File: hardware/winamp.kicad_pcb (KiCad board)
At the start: 2 copper layers, 2.1 x 1.7 mm, 13 parts, among them U101 TLV271QDBVRQ1, U102 ZXBM5210-SP

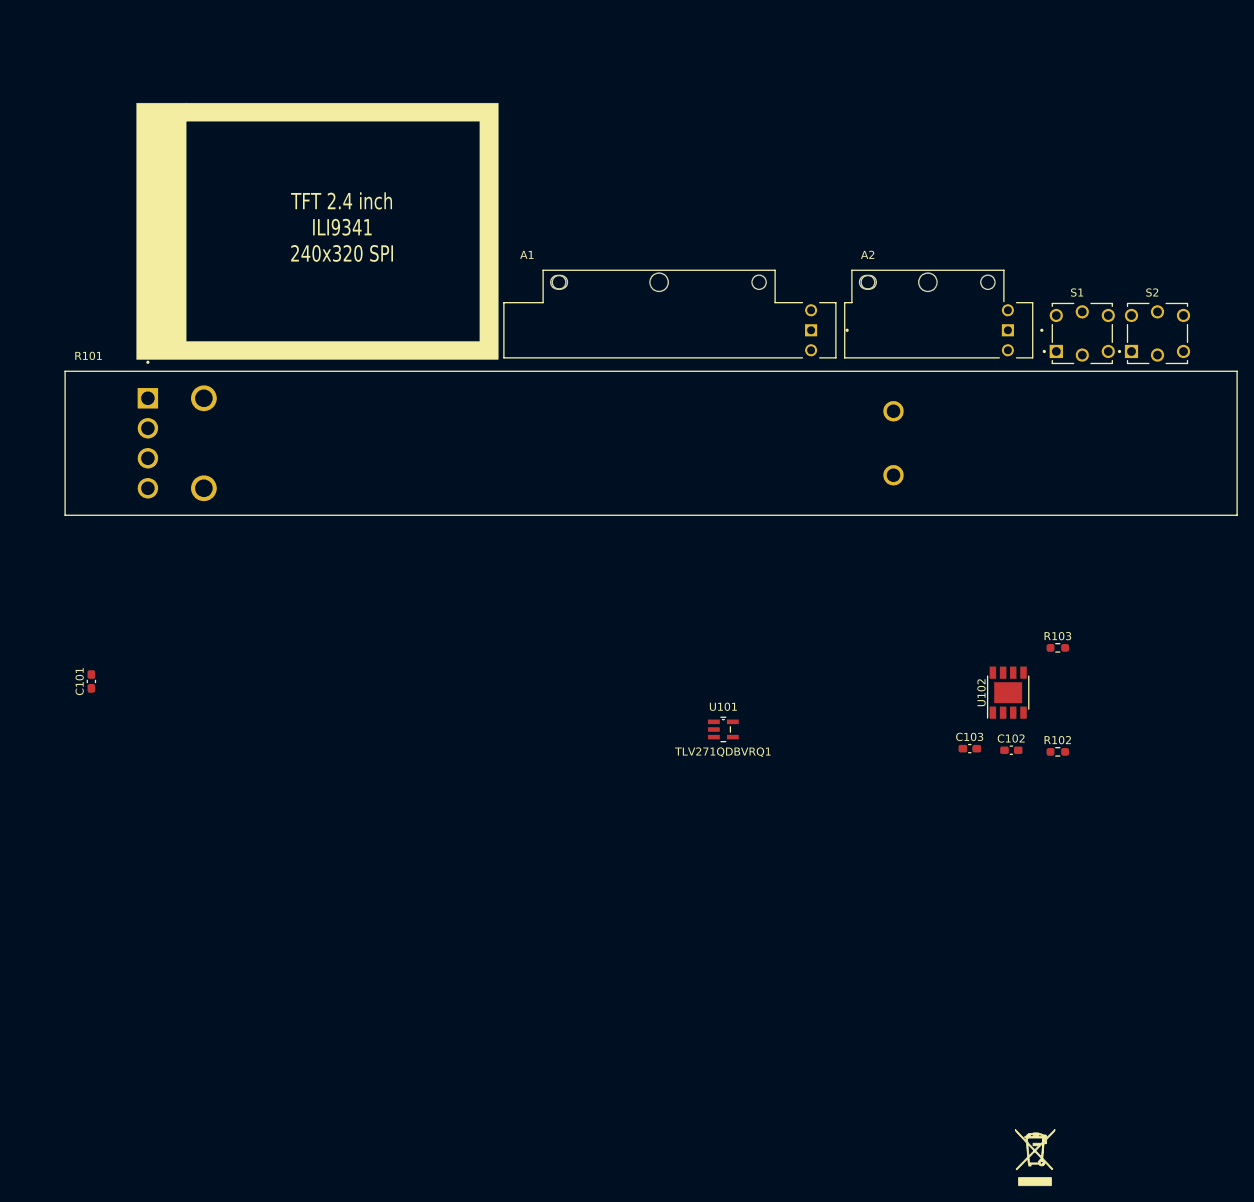
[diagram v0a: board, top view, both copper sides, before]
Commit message: Update winamp.kicad_pcb
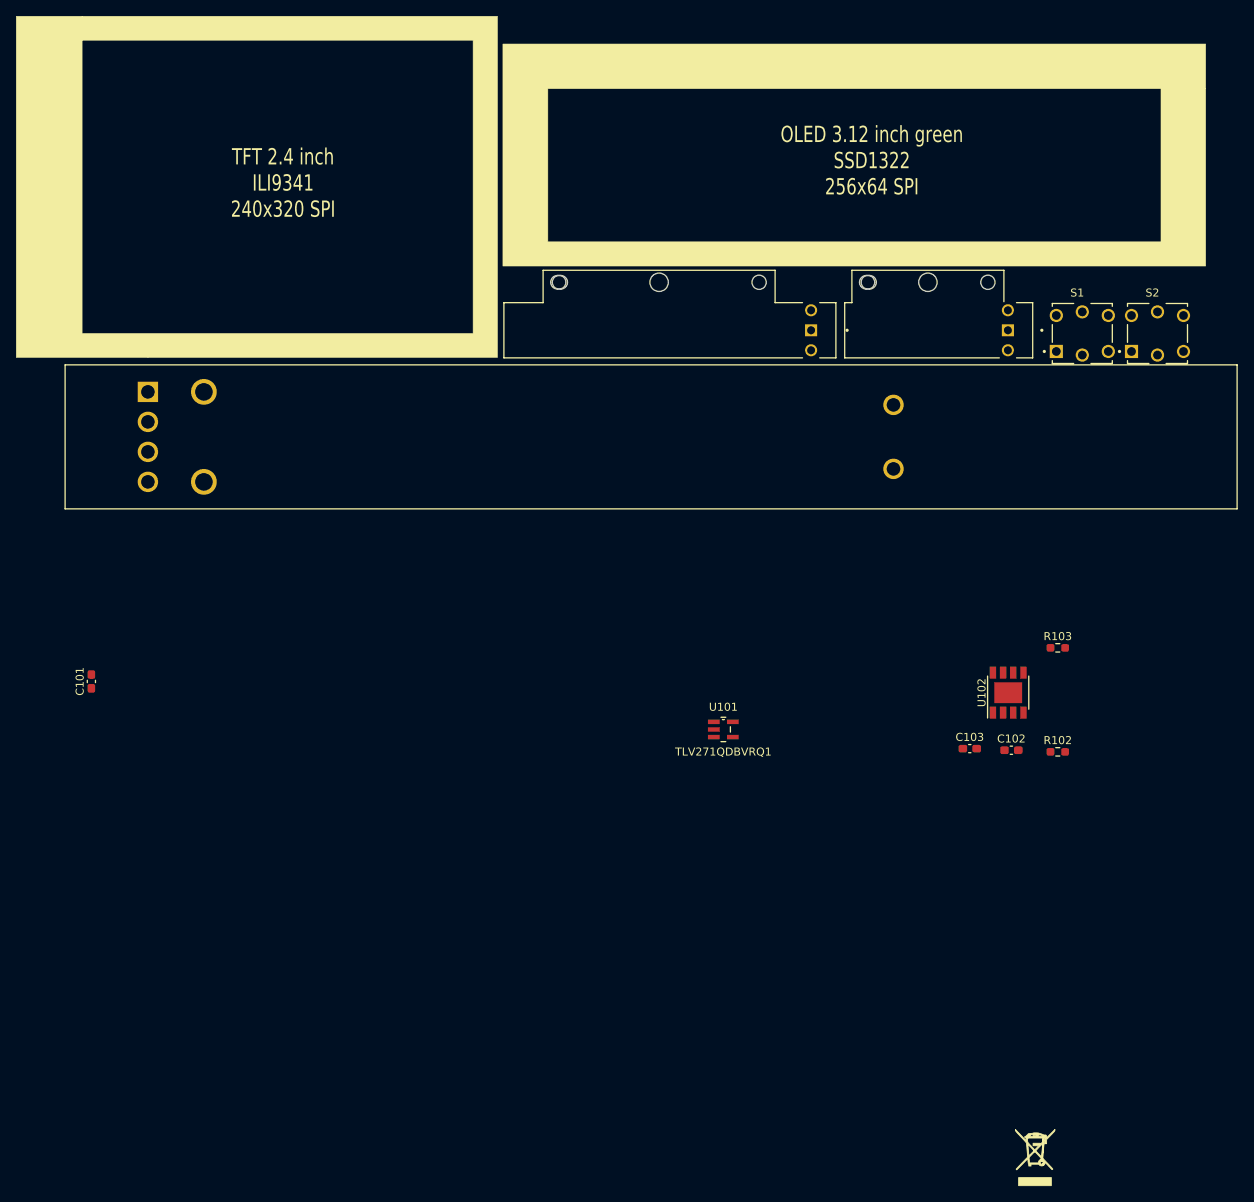
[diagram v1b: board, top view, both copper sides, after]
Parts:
- moved R101 0.80 mm to (116.8, 91.1)
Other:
- board text added: "OLED 3.12 inch green SSD1322 256x64 SPI"
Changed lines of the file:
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@@
   )
   (footprint "RSA0N11M9A07:TRIM_RSA0N11M9A07" (layer "F.Cu")
-    (at 116.8 91.925)
+    (at 116.8 91.125)
     (property "MANUFACTURER" "Alps")
     (property "MAXIMUM_PACKAGE_HEIGHT" "34.70mm")
@@
   (gr_poly
     (pts
-      (xy 52.496229 81.450023)
-      (xy 52.496229 49.410037)
-      (xy 58.680067 49.410037)
-      (xy 58.680067 51.660052)
-      (xy 58.680067 79.2)
-      (xy 95.4 79.2)
-      (xy 95.4 51.660052)
-      (xy 58.680067 51.660052)
-      (xy 58.680067 49.410037)
-      (xy 97.69129 49.410037)
-      (xy 97.69129 81.450023)
-    ) (layer "F.SilkS") (width 0.05) (fill solid))
-  (gr_text "TFT 2.4 inch\nILI9341\n240x320 SPI" (at 78.2 65) (layer "F.SilkS")
+      (xy 98.276965 42.018253)
+      (xy 186.123036 42.018253)
+      (xy 186.123036 47.6)
+      (xy 180.535302 47.6)
+      (xy 103.891826 47.6)
+      (xy 103.891826 66.744498)
+      (xy 180.535302 66.744498)
+      (xy 180.535302 47.6)
+      (xy 186.123036 47.6)
+      (xy 186.123036 69.76955)
+      (xy 98.276965 69.76955)
+    ) (layer "F.SilkS") (width 0.06655) (fill solid))
+  (gr_poly
+    (pts
+      (xy 37.445375 81.194781)
+      (xy 37.445375 38.54956)
+      (xy 45.676063 38.54956)
+      (xy 45.676063 41.54433)
+      (xy 45.676063 78.2)
+      (xy 94.550293 78.2)
+      (xy 94.550293 41.54433)
+      (xy 45.676063 41.54433)
+      (xy 45.676063 38.54956)
+      (xy 97.6 38.54956)
+      (xy 97.6 81.194781)
+    ) (layer "F.SilkS") (width 0.06655) (fill solid))
+  (gr_text "OLED 3.12 inch green\nSSD1322\n256x64 SPI" (at 144.4 56.6) (layer "F.SilkS")
     (effects (font (size 2.032 1.524) (thickness 0.3048)))
   )
-  (group "" (id 70f5c3d3-4adc-47ed-b946-52d46610829d)
+  (gr_text "TFT 2.4 inch\nILI9341\n240x320 SPI" (at 70.8 59.4) (layer "F.SilkS")
+    (effects (font (size 2.032 1.524) (thickness 0.3048)))
+  )
+  (group "" (id 30ead398-6d63-45e0-93e9-14f385270c33)
     (members
-      6dc4ee29-9574-4038-a646-3491c933ab9f
-    )
-  )
+      67b836f5-9abb-410f-a0e0-7620d94d0780
+    )
+  )
+  (group "" (id d69c5e97-8f5a-4b0f-a9a9-389fc3f745f3)
+    (members
+      3cc698f5-0cb1-4cfe-8278-ad0242500876
+    )
+  )

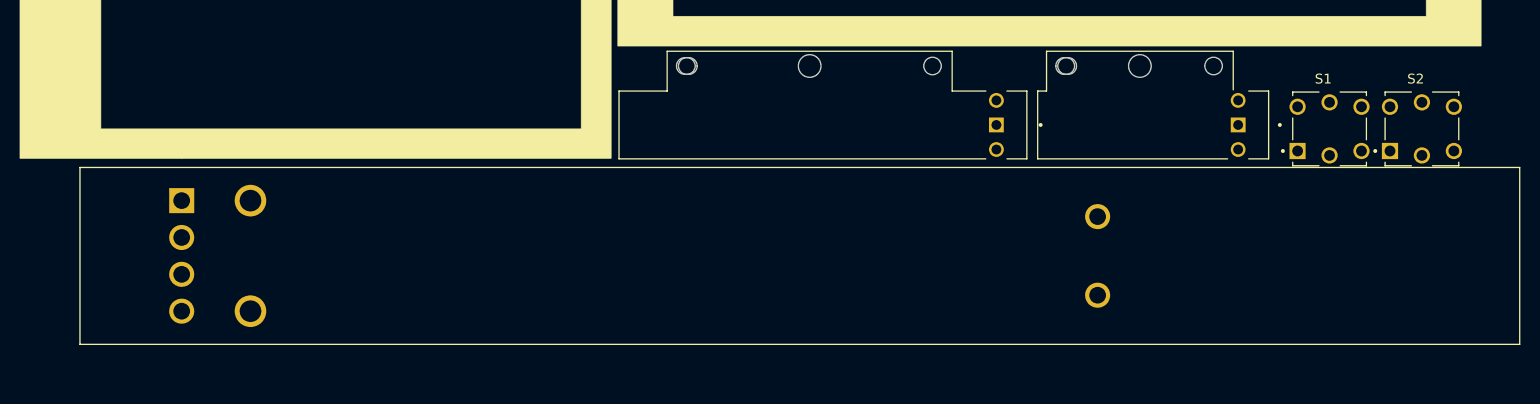
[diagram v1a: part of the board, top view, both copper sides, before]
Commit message: Update winamp.kicad_pcb
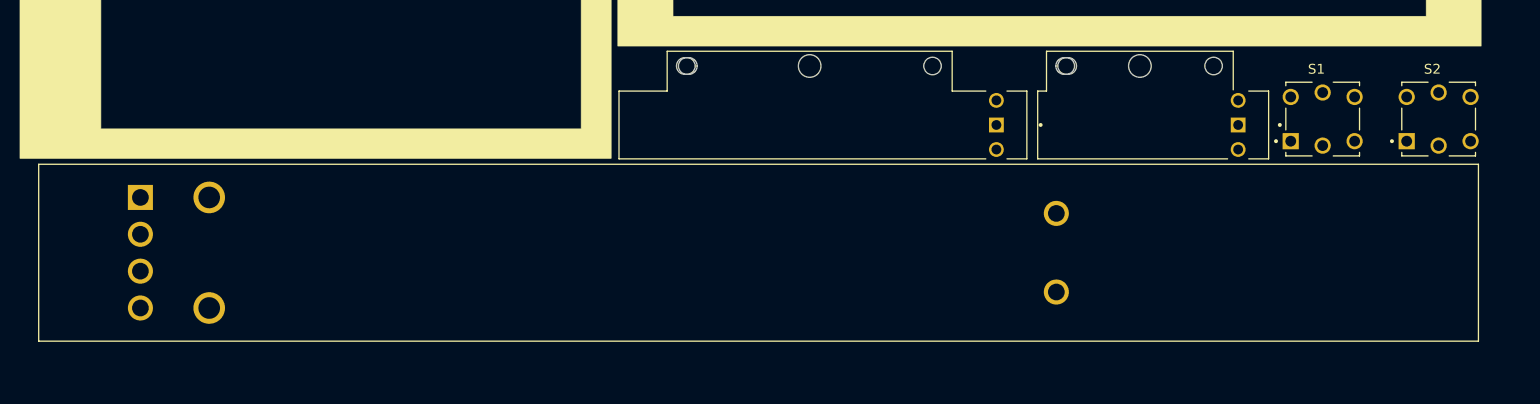
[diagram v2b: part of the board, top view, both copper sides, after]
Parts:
- moved R101 4.21 mm to (112.6, 90.8)
- moved S2 1.97 mm to (181.8, 77.2)
- moved S1 1.22 mm to (170.0, 77.2)
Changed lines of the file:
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@@
   )
   (footprint "TL1240GQ1JCLR:SW_TL1240GQ1JCLR" (layer "F.Cu")
-    (at 170.7 78.2)
+    (at 170 77.2)
     (property "MANUFACTURER" "E-Switch")
     (property "MAXIMUM_PACKAGE_HEIGHT" "7.18.2022")
@@
   )
   (footprint "TL1240GQ1JCLR:SW_TL1240GQ1JCLR" (layer "F.Cu")
-    (at 180.1 78.2)
+    (at 181.8 77.2)
     (property "MANUFACTURER" "E-Switch")
     (property "MAXIMUM_PACKAGE_HEIGHT" "7.18.2022")
@@
       (effects (font (size 1 1) (thickness 0.15)))
     )
-    (fp_text value "TL1240GQ1JCLR" (at 1.9 -7.2) (layer "F.Fab")
+    (fp_text value "TL1240GQ1JCLR" (at 11.4 0) (layer "F.Fab")
       (effects (font (size 1 1) (thickness 0.15)))
     )
@@
   )
   (footprint "RSA0N11M9A07:TRIM_RSA0N11M9A07" (layer "F.Cu")
-    (at 116.8 91.125)
+    (at 112.6 90.8)
     (property "MANUFACTURER" "Alps")
     (property "MAXIMUM_PACKAGE_HEIGHT" "34.70mm")
